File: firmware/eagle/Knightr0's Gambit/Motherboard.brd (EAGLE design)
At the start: 140 x 70 mm, 20 parts, among them IC1 7805T, Q1 BUZ10, X1 22-23-2021, X2 22-23-2031, X3 22-23-2031, X4 22-23-2041, X5 22-23-2041, X6 22-23-2041, X7 22-23-2021, X8 22-23-2021

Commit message: update eagle files
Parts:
- added R7, R8: (no value), rcl:R0603
- added X10, X9: 22-23-2021, con-molex:22-23-2021
- D1: device adafruit:CB417-15 -> adafruit:DO41-10
- moved R6 85.0 mm to (95.2, 75.3), turned to 180 degrees
- moved R5 76.2 mm to (44.5, 75.3)
- moved R4 72.4 mm to (33.0, 75.3)
- moved R1 31.8 mm to (9.78, 72.3)
- moved R3 28.8 mm to (34.3, 47.0), turned to 0 degrees
- moved X8 10.2 mm to (95.2, 81.3)
- moved X7 6.35 mm to (33.0, 81.3)
- moved R2 5.08 mm to (34.3, 52.1), turned to 180 degrees
- moved D1 4.02 mm to (20.3, 72.4)
- moved X5 3.81 mm to (81.3, 81.3)
- moved X6 3.81 mm to (58.4, 81.3)
- moved X2 3.81 mm to (20.3, 81.3)
- moved X1 2.54 mm to (118.1, 81.3)
- moved X3 1.27 mm to (8.89, 66.0)
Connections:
- removed net X_ENDSTOP: BOARD1.D18, R3.1, X7.2
- removed net Y_ENDSTOP: BOARD1.D19, R4.1, X8.2
- new net X_ENDSTOP_MAX: BOARD1.VP, R7.1, X9.2
- new net X_ENDSTOP_MIN: BOARD1.VN, R6.1, X8.2
- new net Y_ENDSTOP_MAX: BOARD1.D34, R5.1, X10.2
- new net Y_ENDSTOP_MIN: BOARD1.D35, R4.1, X7.2
- net +12V: now also R1.2, X2.1; no longer R6.2
- net 3.3V: now also X10.1, X9.1
- net AGND: now also R6.2, R7.2, R8.2; no longer R3.2
- net DRAIN: now also R3.2; no longer R2.2
- net MAGNET: now also R2.1; no longer R1.1
- net N$10: now also R2.2; no longer R1.2
- net N$12: now also R1.1; no longer R6.1, X2.1
- net N$9: now also R3.1; no longer R2.1
- net TIMER_BUTTON: now also R8.1; no longer R5.1
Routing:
- net X_ENDSTOP: track 118.6 -> 0.00 mm
- net Y_ENDSTOP_MIN: track 0.00 -> 87.0 mm
- net Y_ENDSTOP_MAX: track 0.00 -> 74.5 mm
- net Y_ENDSTOP: track 51.5 -> 0.00 mm
- net X_ENDSTOP_MIN: track 0.00 -> 26.4 mm
- net AGND: track 483.2 -> 507.8 mm
- net +12V: track 135.4 -> 156.0 mm
- net X_ENDSTOP_MAX: track 0.00 -> 20.5 mm
- net 3.3V: track 170.5 -> 184.2 mm, vias 2 -> 4
- net N$12: track 18.2 -> 4.66 mm
- net MAGNET: track 122.2 -> 113.8 mm
- net TIMER_BUTTON: track 33.7 -> 36.2 mm
- net N$8: track 51.3 -> 52.9 mm
- net N$6: track 60.7 -> 62.3 mm
- net N$5: track 65.8 -> 67.4 mm
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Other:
- board size 140 x 70 mm -> 142.5 x 70.1 mm
- board text added: "EM"
- board text added: "Power In"
- board text added: "Timer Button"
- board text added: "UART"
- board text added: "X Max"
- board text added: "X Min"
- board text added: "X Motor"
- board text added: "Y Max"
- board text added: "Y Min"
- board text added: "Y Motor"

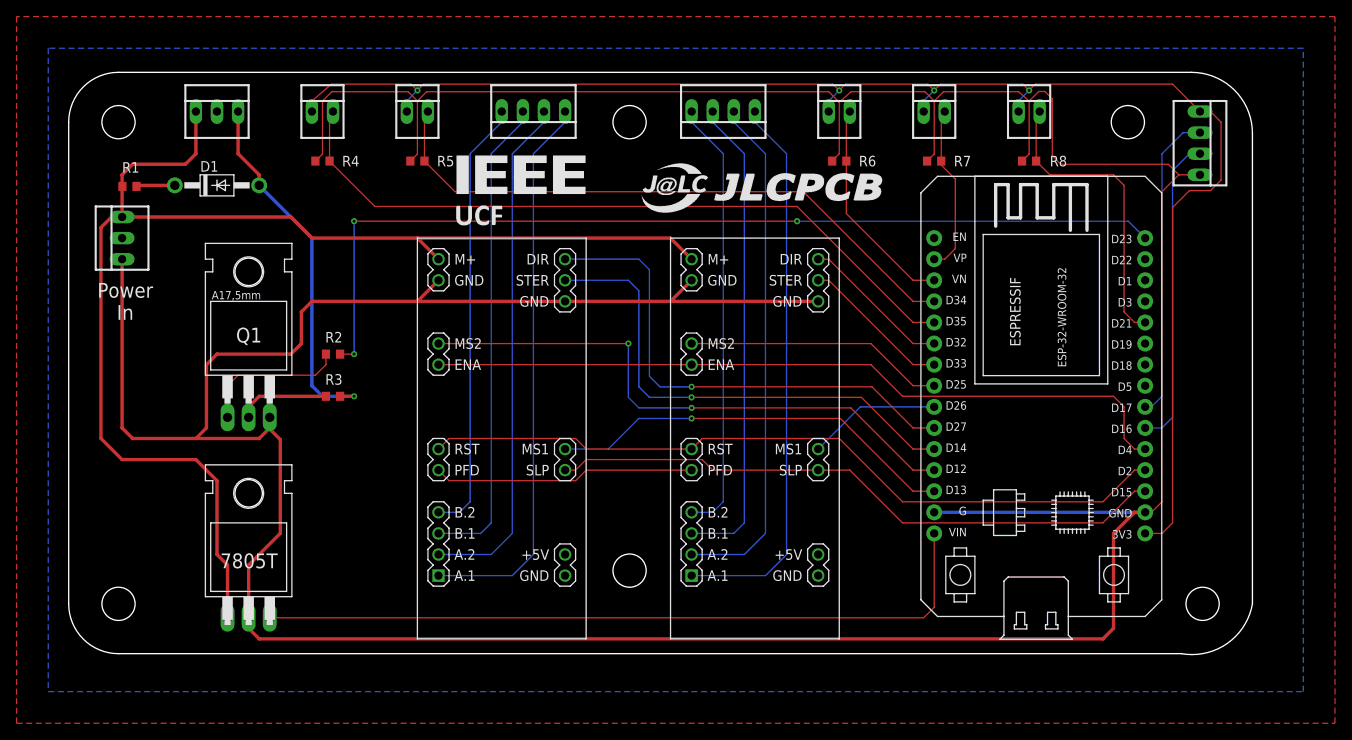
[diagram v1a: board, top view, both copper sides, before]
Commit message: Updated pcb files
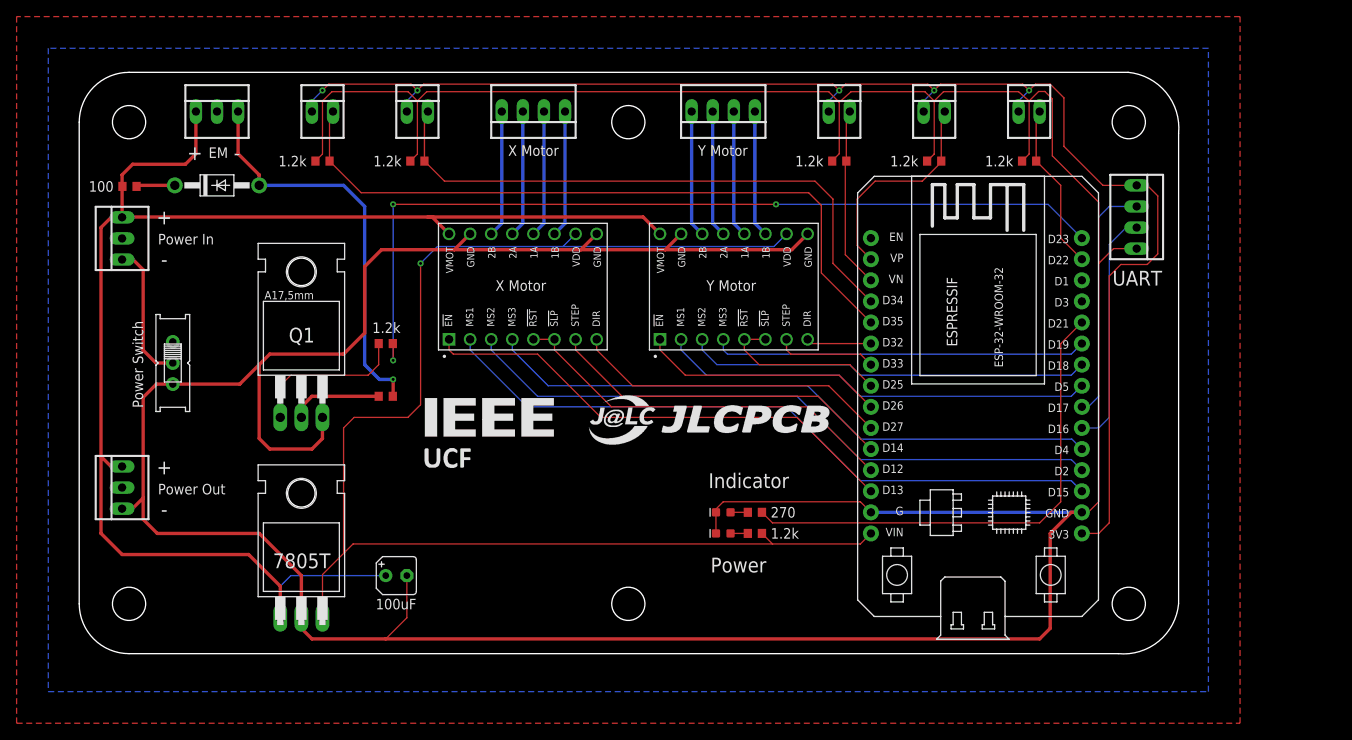
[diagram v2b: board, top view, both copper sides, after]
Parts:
- removed U$1, U$2: STEPPER-MOTOR-EASY-DRIVER, Ultrasonic Sensor:STEPPER-MOTOR-EASY-DRIVER
- added C1: 100uF, rcl:B45181A
- added D2, D3: (no value), SparkFun-LED:LED-0603
- added R10: 270, rcl:R0603
- added R9: 1.2k, rcl:R0603
- added S1: (no value), adafruit:EG1218
- added U1, U2: A4988_STEPPER_MOTOR_DRIVER_CARRIER, A4988_STEPPER_MOTOR_DRIVER_CARRIER:MODULE_A4988_STEPPER_MOTOR_DRIVER_CARRIER
- added X11: 22-23-2031, con-molex:22-23-2031
- R1: value (none) -> 100
- R2, R4, R5, R6, R7, R8: value (none) -> 1.2k
- moved X4 11.7 mm to (131.1, 68.6)
- moved BOARD1 7.62 mm to (124.5, 30.5)
- moved R2 6.48 mm to (40.6, 53.3)
- moved IC1 6.35 mm to (30.5, 30.5)
- moved Q1 6.35 mm to (30.5, 50.8)
- moved R3 6.35 mm to (40.6, 47.0)
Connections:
- removed net ENA: BOARD1.D4, U$1.JP6.1, U$2.JP6.1
- removed net PFD: U$1.JP7.1, U$2.JP7.1
- removed net RST: BOARD1.D2, U$1.JP7.2, U$2.JP7.2
- removed net SLP: BOARD1.D15, U$1.JP5.2, U$2.JP5.2
- new net INDICATOR_LED: BOARD1.D21, R10.2
- new net N$13: S1.P, X3.1
- new net N$22: U1.13, X6.3
- new net N$23: U1.14, X6.4
- new net X_ENA: BOARD1.D13, U1.1
- new net X_MS3: BOARD1.D4, U1.4
- new net X_SLP/RST: BOARD1.D12, U1.5, U1.6
- new net Y_ENA: BOARD1.D26, U2.1
- new net Y_MS3: BOARD1.D19, U2.4
- new net Y_SLP/RST: BOARD1.D25, U2.5, U2.6
- net +12V: now also C1.+, U1.16, U2.16, X11.3; no longer U$1.JP1.2, U$2.JP1.2
- net +5V: now also R9.2, U1.10, U2.10
- net AGND: now also C1.-, D2.C, D3.C, S1.S, U1.15, U1.9, U2.15, U2.9, X11.1; no longer U$1.JP1.1, U$1.JP2.1, U$2.JP1.1, U$2.JP2.1, X3.1
- net N$1: now also U2.12, X5.2; no longer U$1.JP3.1, X6.1
- net N$2: now also U2.11, X5.1; no longer U$1.JP3.2, X6.2
- net N$3: now also U2.13, X5.3; no longer U$1.JP3.3, X6.3
- net N$4: now also U2.14, X5.4; no longer U$1.JP3.4, X6.4
- net N$5: now also U1.12, X6.2; no longer U$2.JP3.1, X5.1
- net N$6: now also U1.11, X6.1; no longer U$2.JP3.2, X5.2
- net N$7: now also D2.A, R9.1; no longer U$2.JP3.3, X5.3
- net N$8: now also D3.A, R10.1; no longer U$2.JP3.4, X5.4
- net TIMER_BUTTON: now also BOARD1.D22; no longer BOARD1.D21
- net X_DIR: now also U1.8; no longer U$1.JP2.3
- net X_MS1: now also BOARD1.D15, U1.2; no longer BOARD1.D13, U$1.JP5.1
- net X_MS2: now also BOARD1.D2, U1.3; no longer BOARD1.D12, U$1.JP6.2
- net X_STEP: now also U1.7; no longer U$1.JP2.2
- net Y_DIR: now also U2.8; no longer U$2.JP2.3
- net Y_MS1: now also BOARD1.D5, U2.2; no longer BOARD1.D26, U$2.JP5.1
- net Y_MS2: now also BOARD1.D18, U2.3; no longer BOARD1.D25, U$2.JP6.2
- net Y_STEP: now also U2.7; no longer U$2.JP2.2
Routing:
- net ENA: track 91.5 -> 0.00 mm
- net RST: track 91.4 -> 0.00 mm
- net +5V: track 89.4 -> 165.4 mm, vias 0 -> 1
- net SLP: track 75.1 -> 0.00 mm
- net X_MS3: track 0.00 -> 74.8 mm
- net INDICATOR_LED: track 0.00 -> 60.2 mm
- net X_ENA: track 0.00 -> 59.1 mm
- net N$7: track 58.0 -> 2.08 mm
- net N$5: track 67.4 -> 15.3 mm
- net N$1: track 67.4 -> 15.3 mm
- net N$8: track 52.9 -> 2.11 mm
- net X_SLP/RST: track 0.00 -> 47.9 mm
- net N$6: track 62.3 -> 15.3 mm
- net N$2: track 62.3 -> 15.3 mm
- net Y_MS3: track 0.00 -> 45.2 mm
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- added copper zone on layer 1, net AGND
- added copper zone on layer 16, net AGND
- removed copper zone on layer 1, net GND
- removed copper zone on layer 16, net GND
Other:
- board size 142.5 x 70.1 mm -> 132.4 x 70 mm
- board text added: "+"
- board text added: "-"
- board text added: "Indicator"
- board text added: "Power"
- board text added: "Power Out"
- board text added: "Power Switch"
